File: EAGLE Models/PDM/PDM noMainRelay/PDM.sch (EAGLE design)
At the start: 20 parts

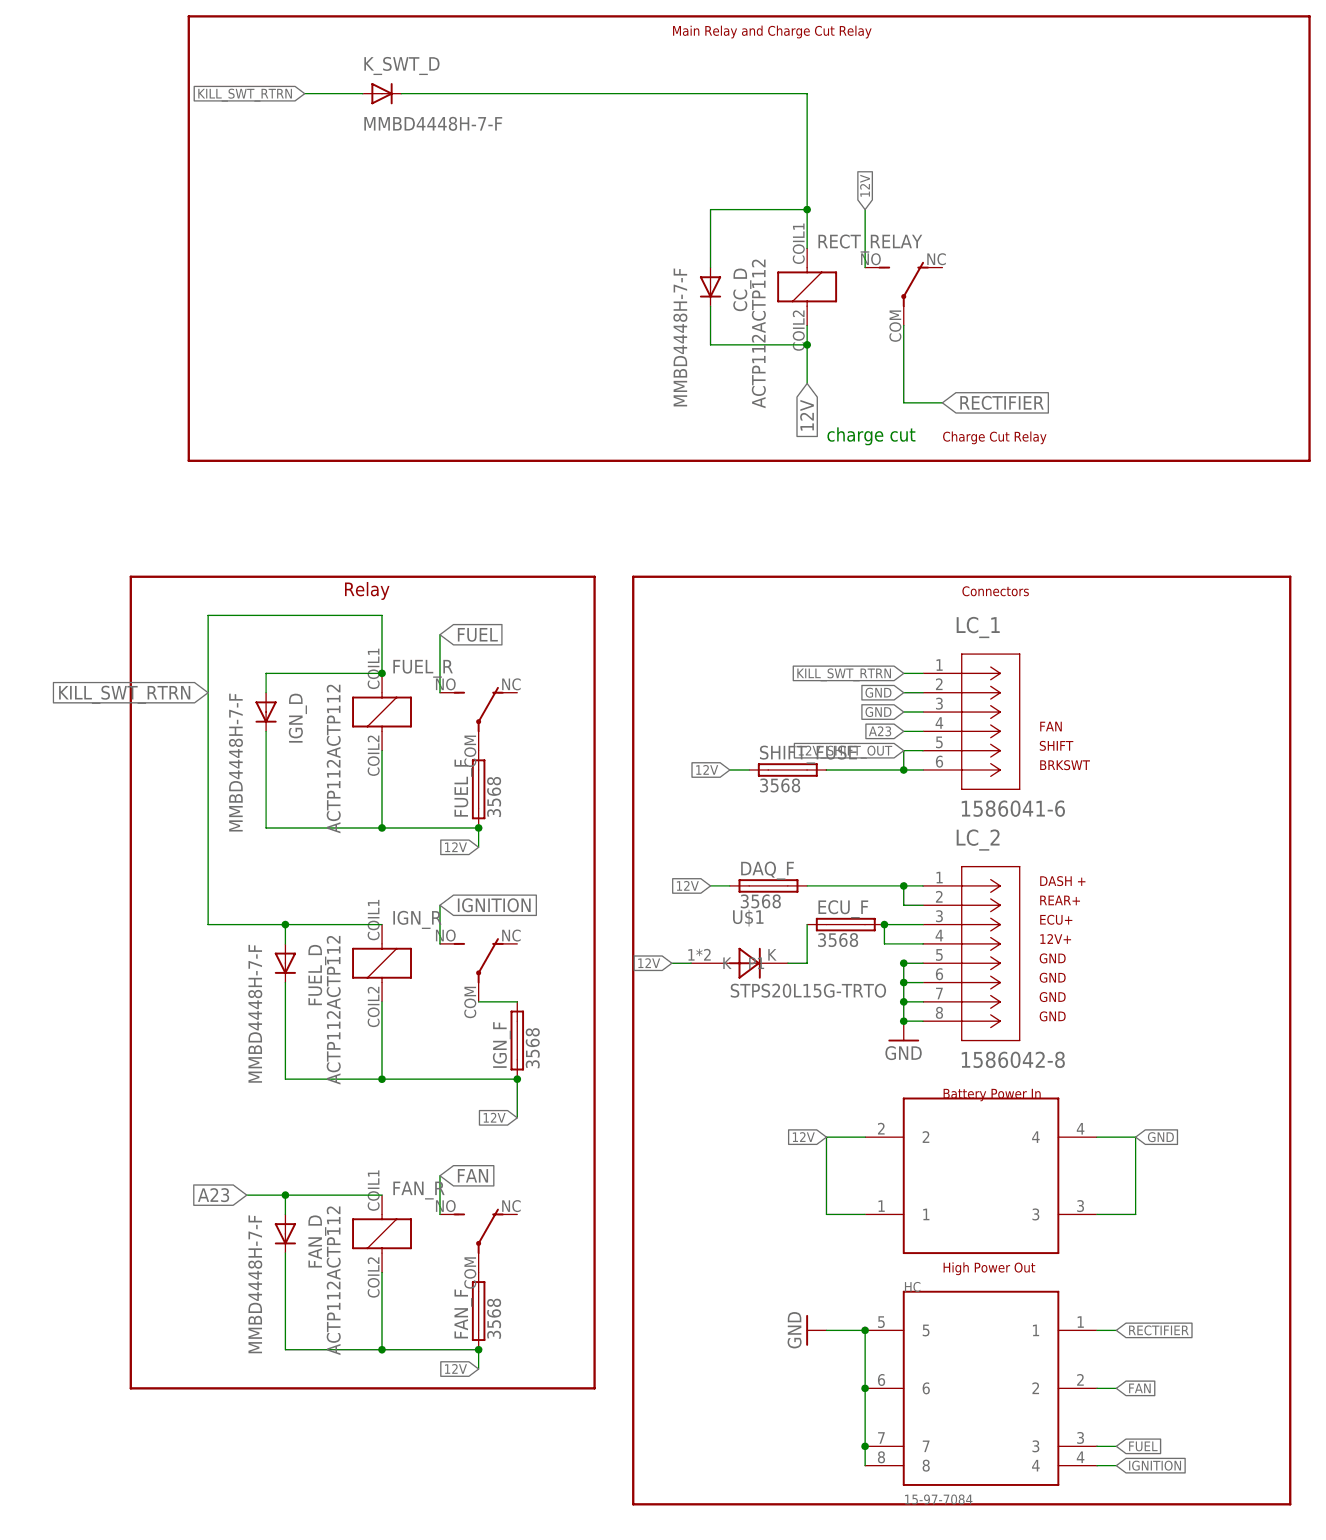
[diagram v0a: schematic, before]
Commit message: C-Car PDM
Assigned Pin Connections
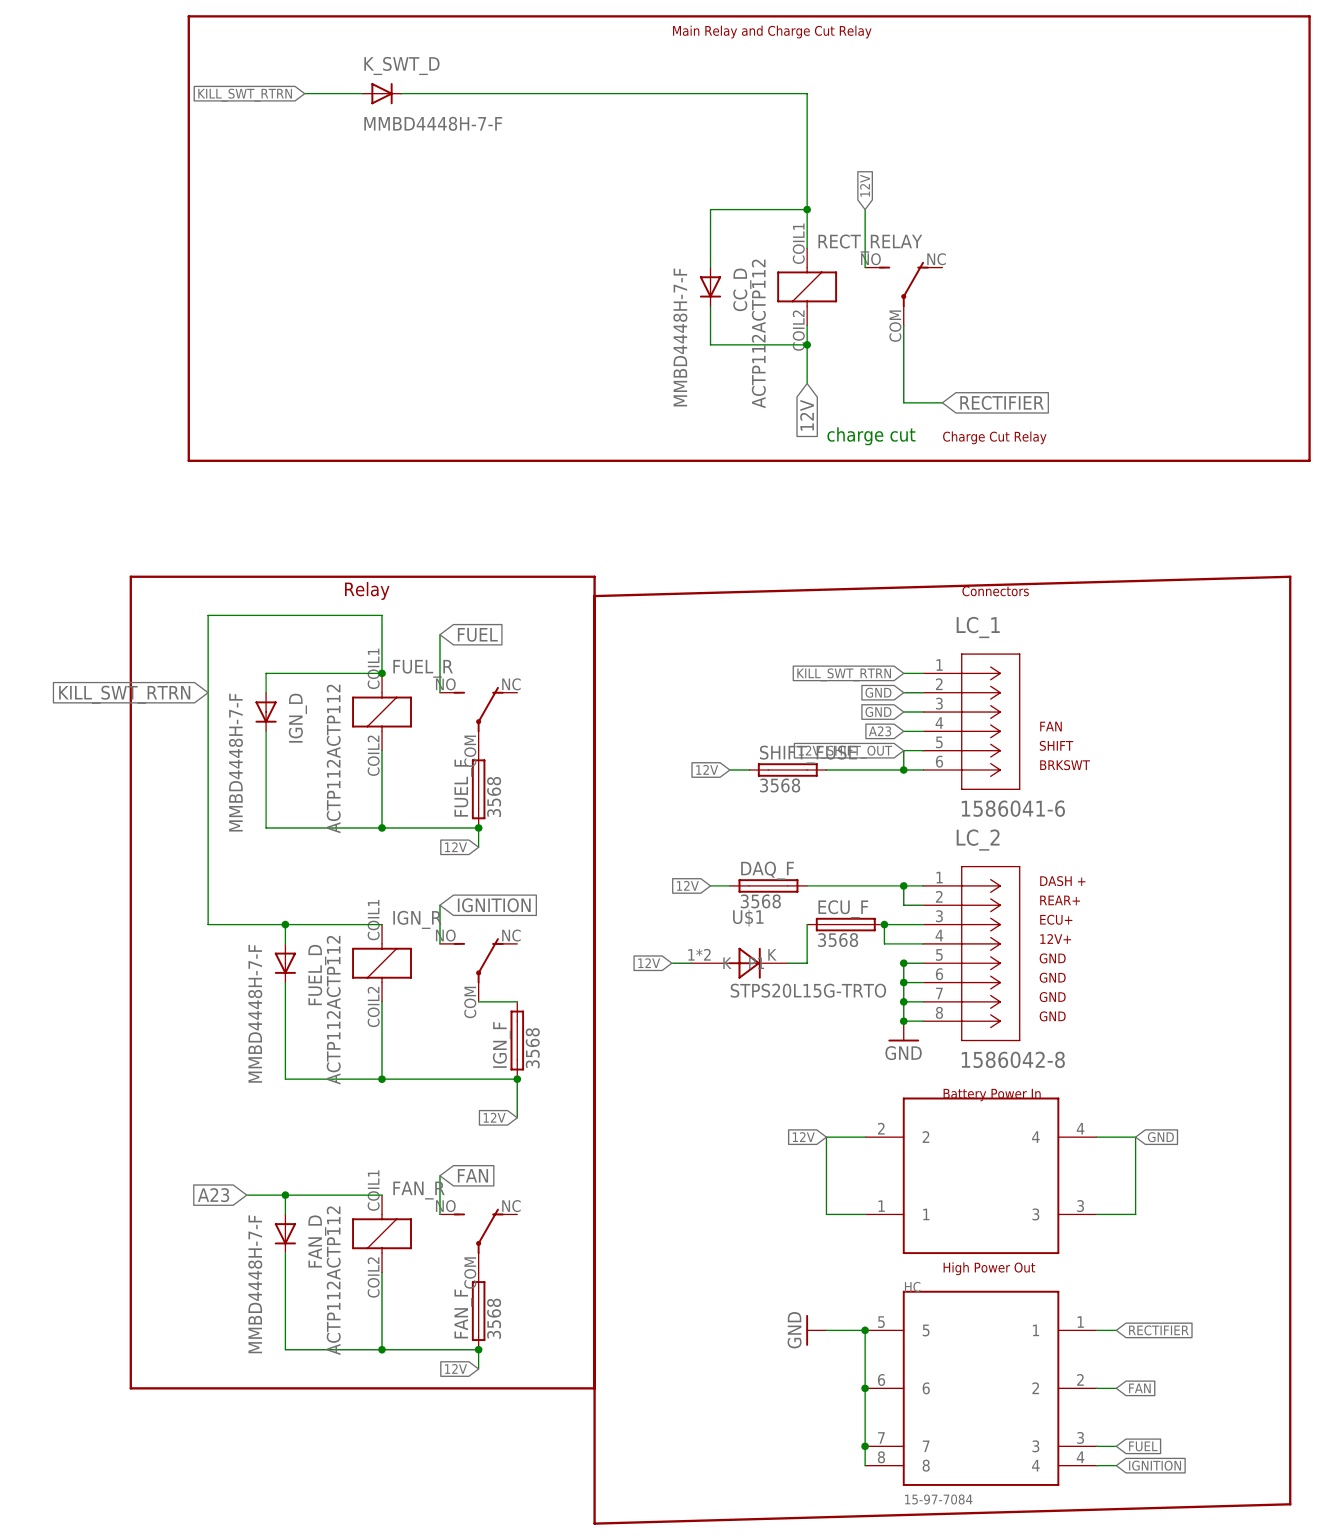
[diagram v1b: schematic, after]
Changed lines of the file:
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@@
 <?xml version="1.0" encoding="utf-8"?>
 <!DOCTYPE eagle SYSTEM "eagle.dtd">
-<eagle version="7.7.0">
+<eagle version="8.3.2">
 <drawing>
 <settings>
 <setting alwaysvectorfont="no"/>
+<setting keepoldvectorfont="yes"/>
 <setting verticaltext="up"/>
 </settings>
@@
 <text x="48.26" y="-30.48" size="1.27" layer="94">BRKSWT</text>
 <text x="35.56" y="12.7" size="1.27" layer="94">Charge Cut Relay</text>
-<wire x1="-5.08" y1="-5.08" x2="-5.08" y2="-127" width="0.3048" layer="94"/>
-<wire x1="-5.08" y1="-127" x2="81.28" y2="-127" width="0.3048" layer="94"/>
+<wire x1="-10.16" y1="-7.62" x2="-10.16" y2="-129.54" width="0.3048" layer="94"/>
+<wire x1="-10.16" y1="-129.54" x2="81.28" y2="-127" width="0.3048" layer="94"/>
 <wire x1="81.28" y1="-127" x2="81.28" y2="-5.08" width="0.3048" layer="94"/>
-<wire x1="81.28" y1="-5.08" x2="-5.08" y2="-5.08" width="0.3048" layer="94"/>
+<wire x1="81.28" y1="-5.08" x2="-10.16" y2="-7.62" width="0.3048" layer="94"/>
 <text x="38.1" y="-7.62" size="1.27" layer="94">Connectors</text>
 <text x="35.56" y="-73.66" size="1.27" layer="94">Battery Power In</text>
